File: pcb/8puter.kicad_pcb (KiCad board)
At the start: 2 copper layers, 120 x 100 mm, 72 parts, among them J1 PWR-DC, U1 74AC00, U2 74AHC74, U3 74HC126, U6 MAX811TEUS+T, X1 ECS-2200BX-100

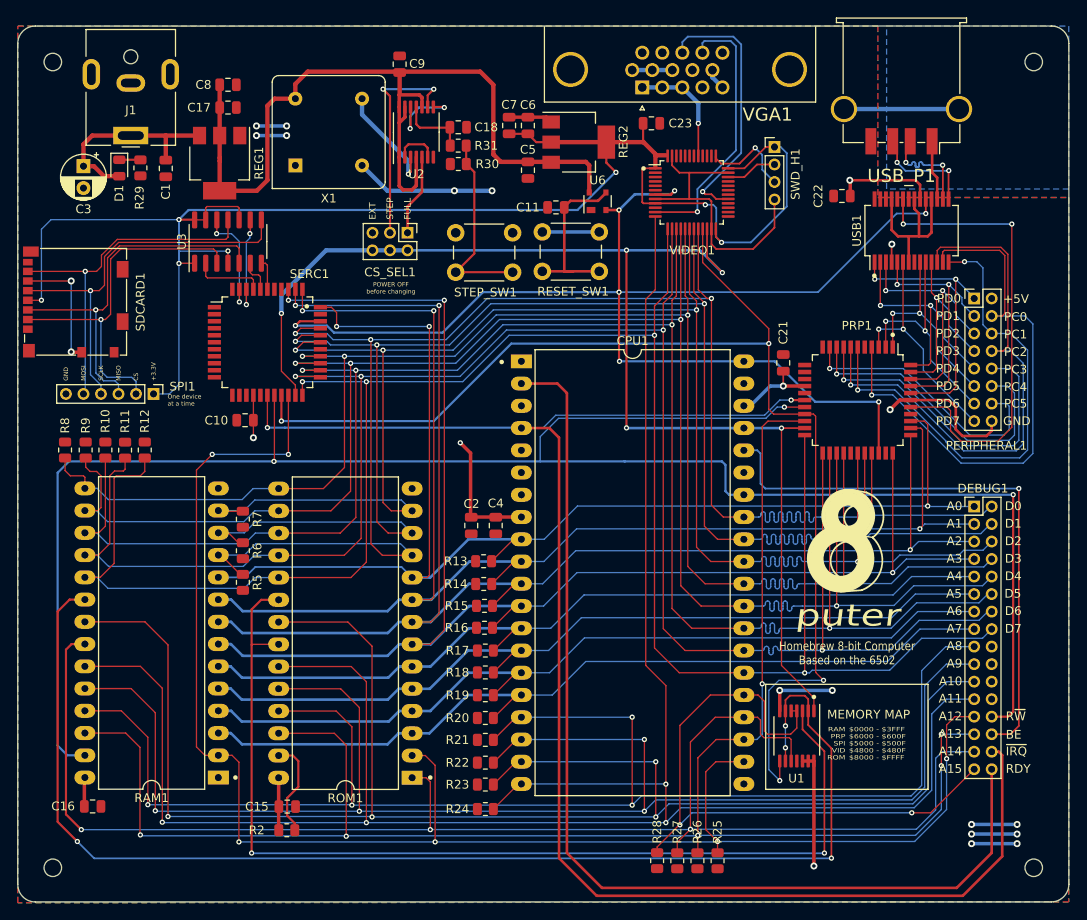
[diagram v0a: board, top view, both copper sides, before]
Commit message: Clearances
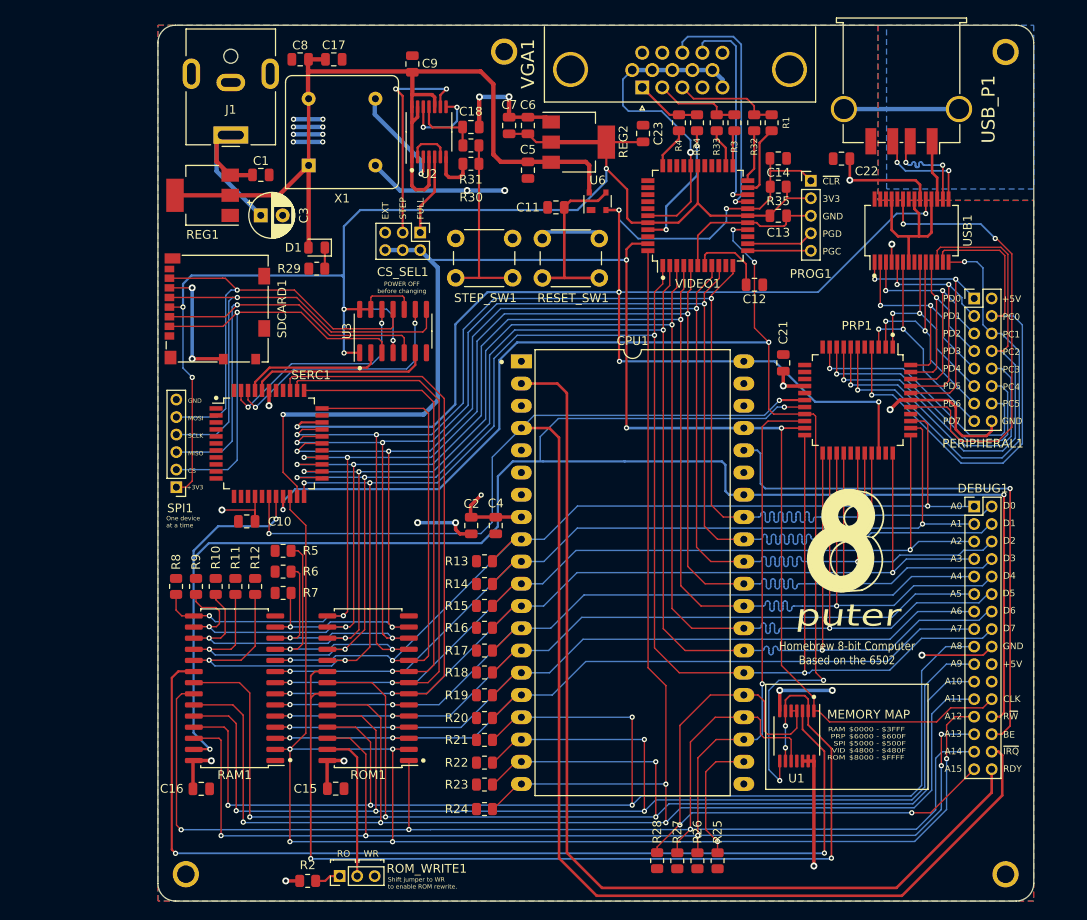
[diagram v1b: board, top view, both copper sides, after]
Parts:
- removed SWD_H1: Conn_01x04, Connector_PinHeader_2.00mm:PinHeader_1x04_P2.00mm_Vertical
- added ?: , , F.Cu at (107.9, 132.1)
- added ?: , , F.Cu at (201.5, 132.1)
- added ?: , , F.Cu at (201.5, 38.2)
- added ?: , , F.Cu at (144.2, 38.2)
- added C12: 10uF, Capacitor_SMD:C_0805_2012Metric, F.Cu at (172.8, 64.8)
- added C13: 100nF, Capacitor_SMD:C_0805_2012Metric, F.Cu at (175.5, 56.9)
- added C14: 100nF, Capacitor_SMD:C_0805_2012Metric, F.Cu at (175.5, 50.4)
- added PROG1: Conn_01x05, Connector_PinHeader_2.00mm:PinHeader_1x05_P2.00mm_Vertical, F.Cu at (179.2, 52.9)
- added R1: 1K, Resistor_SMD:R_0805_2012Metric, F.Cu at (174.8, 46.3)
- added R3: 1K, Resistor_SMD:R_0805_2012Metric, F.Cu at (170.5, 46.3)
- added R32: 470R, Resistor_SMD:R_0805_2012Metric, F.Cu at (172.8, 46.3)
- added R33: 470R, Resistor_SMD:R_0805_2012Metric, F.Cu at (168.5, 46.3)
- added R34: 470R, Resistor_SMD:R_0805_2012Metric, F.Cu at (166.2, 46.3)
- added R35: 10K, Resistor_SMD:R_0805_2012Metric, F.Cu at (175.5, 53.6)
- added R4: 1K, Resistor_SMD:R_0805_2012Metric, F.Cu at (164.2, 46.3)
- added ROM_WRITE1: Conn_01x03, Connector_PinHeader_2.00mm:PinHeader_1x03_P2.00mm_Vertical, F.Cu at (125.4, 132.3)
- C11: value 10nF -> 100nF
- R29: value 1.5K -> 1K
- RAM1: value AS6C62256-55PCN -> AS6C62256-55SINTR; footprint Package_DIP:DIP-28_W15.24mm_LongPads -> Package_SO:SOIC-28W_7.5x17.9mm_P1.27mm
- ROM1: value AT28C256 -> AT28HC256E-90SU; footprint Package_DIP:DIP-28_W15.24mm_LongPads -> Package_SO:SOIC-28W_7.5x17.9mm_P1.27mm
- VIDEO1: value STM32F301C8T6 -> PIC32MX270F256D; footprint Package_QFP:TQFP-48_7x7mm_P0.5mm -> Package_QFP:TQFP-44_10x10mm_P0.8mm
- moved D1 24.3 mm to (122.8, 60.5), turned to 180 degrees
- moved R29 23.2 mm to (122.8, 62.9), turned to 180 degrees
- moved U3 21.4 mm to (131.5, 70.1)
- moved C3 21.0 mm to (116.4, 56.9), turned to 0 degrees
- moved R8 20.1 mm to (106.8, 99.2)
- moved R12 20.0 mm to (115.8, 99.2)
- moved R10 20.0 mm to (111.3, 99.2)
- moved R9 20.0 mm to (109.0, 99.2)
- moved R11 20.0 mm to (113.5, 99.2)
- moved SDCARD1 16.2 mm to (111.5, 67.5)
- moved C17 13.3 mm to (124.8, 39.0)
- moved C16 12.6 mm to (109.6, 122.3)
- moved C10 11.6 mm to (114.8, 91.8)
- moved SERC1 11.6 mm to (117.4, 82.9)
- moved J1 11.4 mm to (113.0, 47.7)
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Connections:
- D1 pad 2: /Power/PWR -> +5V
- DEBUG1 pad 18: unconnected-(DEBUG1-Pad18) -> GND
- DEBUG1 pad 20: unconnected-(DEBUG1-Pad20) -> +5V
- DEBUG1 pad 24: unconnected-(DEBUG1-Pad24) -> CLOCK
- R2 pad 2: Net-(ROM1-Pad27) -> Net-(R2-Pad2)
- RAM1 pad 20: ~{ROM_CS} -> ~{RAM_CS}
- ROM1 pad 20: ~{RAM_CS} -> ~{ROM_CS}
- ROM1 pad 22: ~{RAM_CS} -> ~{ROM_CS}
- VGA1 pad 1: /Video/COLOR -> /Video/RED
- VGA1 pad 2: /Video/COLOR -> /Video/GREEN
- VGA1 pad 3: /Video/COLOR -> /Video/BLUE
- VGA1 pad 9: unconnected-(VGA1-Pad9) -> GND
- VIDEO1 pad 1: +3V3 -> DATA7
- VIDEO1 pad 11: /Video/VSYNC -> DATA0
- VIDEO1 pad 12: ADDR11 -> Net-(PROG1-Pad5)
- VIDEO1 pad 13: DATA7 -> Net-(PROG1-Pad4)
- VIDEO1 pad 14: DATA6 -> unconnected-(VIDEO1-Pad14)
- VIDEO1 pad 15: DATA5 -> ~{PRP_CS}
- VIDEO1 pad 16: DATA4 -> GND
- VIDEO1 pad 17: DATA3 -> +3V3
- VIDEO1 pad 18: DATA2 -> ~{RESET}
- VIDEO1 pad 19: DATA1 -> /Video/HSYNC
- VIDEO1 pad 2: unconnected-(VIDEO1-Pad2) -> DATA6
- VIDEO1 pad 20: DATA0 -> /Video/VSYNC
- VIDEO1 pad 21: ~{PRP_CS} -> Net-(VIDEO1-Pad21)
- VIDEO1 pad 22: CLOCK -> Net-(VIDEO1-Pad22)
- VIDEO1 pad 23: GND -> Net-(VIDEO1-Pad23)
- VIDEO1 pad 24: +3V3 -> Net-(R33-Pad2)
- VIDEO1 pad 28: unconnected-(VIDEO1-Pad28) -> +3V3
- VIDEO1 pad 29: /Video/HSYNC -> GND
- VIDEO1 pad 3: unconnected-(VIDEO1-Pad3) -> DATA5
- VIDEO1 pad 33: unconnected-(VIDEO1-Pad33) -> Net-(VIDEO1-Pad33)
- VIDEO1 pad 34: Net-(SWD_H1-Pad2) -> unconnected-(VIDEO1-Pad34)
- VIDEO1 pad 35: GND -> unconnected-(VIDEO1-Pad35)
- VIDEO1 pad 36: +3V3 -> unconnected-(VIDEO1-Pad36)
- VIDEO1 pad 37: Net-(SWD_H1-Pad3) -> unconnected-(VIDEO1-Pad37)
- VIDEO1 pad 39: unconnected-(VIDEO1-Pad39) -> GND
- VIDEO1 pad 4: unconnected-(VIDEO1-Pad4) -> DATA4
- VIDEO1 pad 40: unconnected-(VIDEO1-Pad40) -> +3V3
- VIDEO1 pad 41: /Video/COLOR -> Net-(R34-Pad2)
- VIDEO1 pad 43: unconnected-(VIDEO1-Pad43) -> CLOCK
- VIDEO1 pad 44: unconnected-(VIDEO1-Pad44) -> ADDR11
- VIDEO1 pad 5: unconnected-(VIDEO1-Pad5) -> DATA3
- VIDEO1 pad 6: unconnected-(VIDEO1-Pad6) -> GND
- VIDEO1 pad 7: ~{RESET} -> Net-(C12-Pad1)
- VIDEO1 pad 8: GND -> DATA2
- VIDEO1 pad 9: +3V3 -> DATA1
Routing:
- net GND: track 166.8 -> 201.1 mm, vias 17 -> 22
- net ~{ROM_CS}: track 146.9 -> 113.8 mm
- net ~{RESET}: track 148.4 -> 179.6 mm
- net ADDR11: track 247.2 -> 218.5 mm
- net ADDR10: track 191.8 -> 163.2 mm
- net CLOCK: track 145.8 -> 171.9 mm, vias 5 -> 4
- net +3V3: track 193.4 -> 169.6 mm, vias 7 -> 6
- net ADDR9: track 176.1 -> 155.2 mm
- net ADDR8: track 170.6 -> 152.6 mm
- net ADDR14: track 171.1 -> 153.6 mm
- net Net-(SERC1-Pad42): track 11.6 -> 28.6 mm
- net Net-(SERC1-Pad40): track 3.87 -> 20.7 mm
- net ADDR13: track 200.3 -> 184.0 mm
- net ADDR12: track 186.3 -> 171.1 mm
- net DATA7: track 234.9 -> 219.9 mm, vias 4 -> 6
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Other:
- board size 120 x 100 mm -> 100 x 100 mm
- board text added: "+3V3"
- board text added: "3V3"
- board text added: "CLK"
- board text added: "PGC"
- board text added: "PGD"
- board text added: "RO"
- board text added: "Shift jumper to WR to enable ROM rewrite."
- board text added: "WR"
- board text added: "~{CLR}"
- board text removed: "+3.3V"
